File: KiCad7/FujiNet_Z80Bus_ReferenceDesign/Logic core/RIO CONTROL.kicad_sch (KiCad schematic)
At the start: 8 parts, among them IC1 74HC32N, IC2 7404N, IC4 74HC08N, IC8 74HC32N, IC9 74HC08N

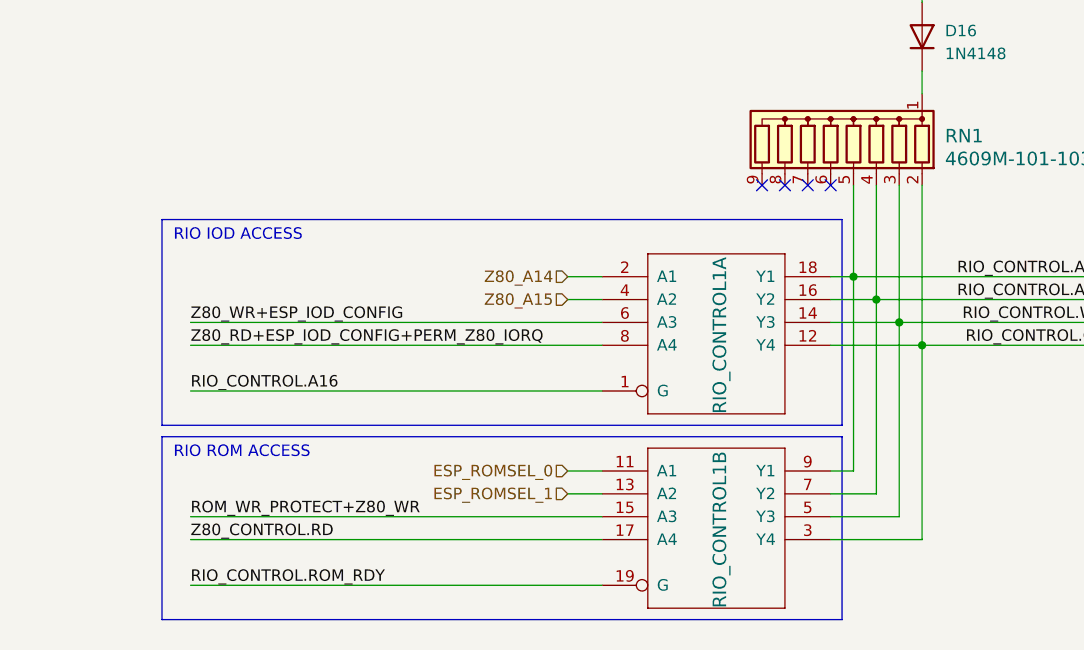
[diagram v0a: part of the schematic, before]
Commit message: KiCad - ALMOST ERROR FREE!!!!
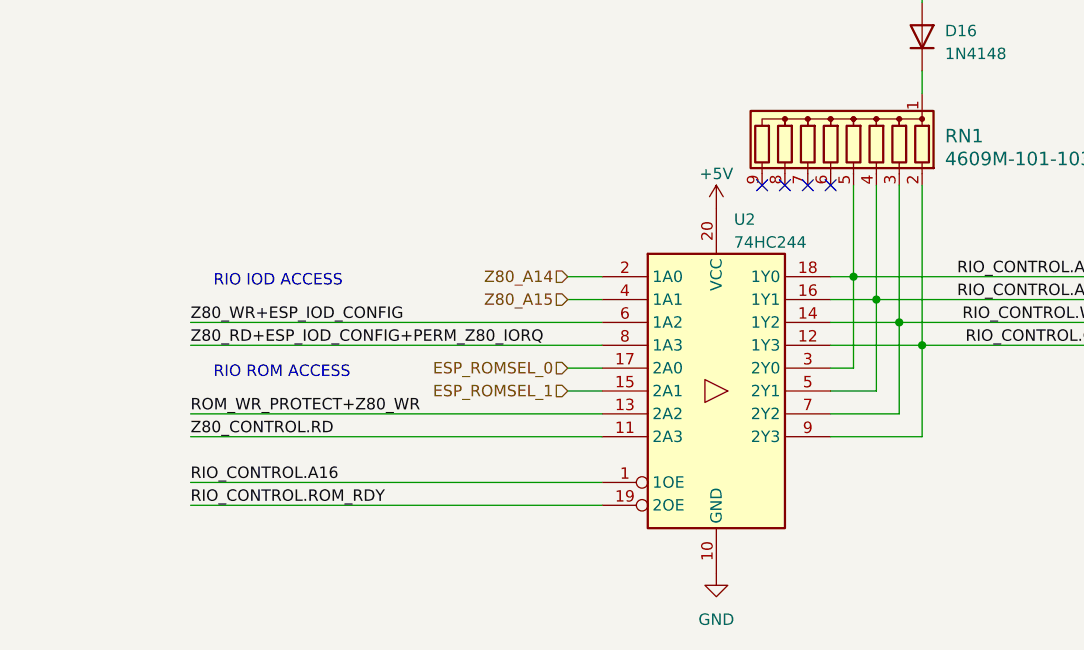
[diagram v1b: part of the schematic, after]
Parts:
- removed RIO_CONTROL1: 74244N, Package_DIP:DIP-20_W7.62mm_Socket, symbol FujiNet_Z80Bus_Reference-rescue:74244N-Z80Decoder-eagle-import
- added U2: 74HC244, symbol 74xx:74HC244
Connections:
- net +5V: now also U2.20 (VCC)
- net ESP_ROMSEL_0: now also U2.17 (2A0)
- net ESP_ROMSEL_1: now also U2.15 (2A1)
- net RIO_CONTROL.A14: now also U2.18 (1Y0), U2.3 (2Y0)
- net RIO_CONTROL.A15: now also U2.16 (1Y1), U2.5 (2Y1)
- net RIO_CONTROL.A16: now also U2.1 (1OE)
- net RIO_CONTROL.OE: now also U2.12 (1Y3), U2.9 (2Y3)
- net RIO_CONTROL.ROM_RDY: now also U2.19 (2OE)
- net RIO_CONTROL.WE: now also U2.14 (1Y2), U2.7 (2Y2)
- net ROM_WR_PROTECT+Z80_WR: now also U2.13 (2A2)
- net Z80_A14: now also U2.2 (1A0)
- net Z80_A15: now also U2.4 (1A1)
- net Z80_CONTROL.RD: now also U2.11 (2A3)
- net Z80_RD+ESP_IOD_CONFIG+PERM_Z80_IORQ: now also U2.8 (1A3)
- net Z80_WR+ESP_IOD_CONFIG: now also U2.6 (1A2)
- new net GND: U2.10 (GND)
